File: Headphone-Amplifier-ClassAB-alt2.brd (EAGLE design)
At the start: 40.6 x 17.8 mm, 17 parts, among them T1 2N3904, T2 2N3904, T3 2N3906

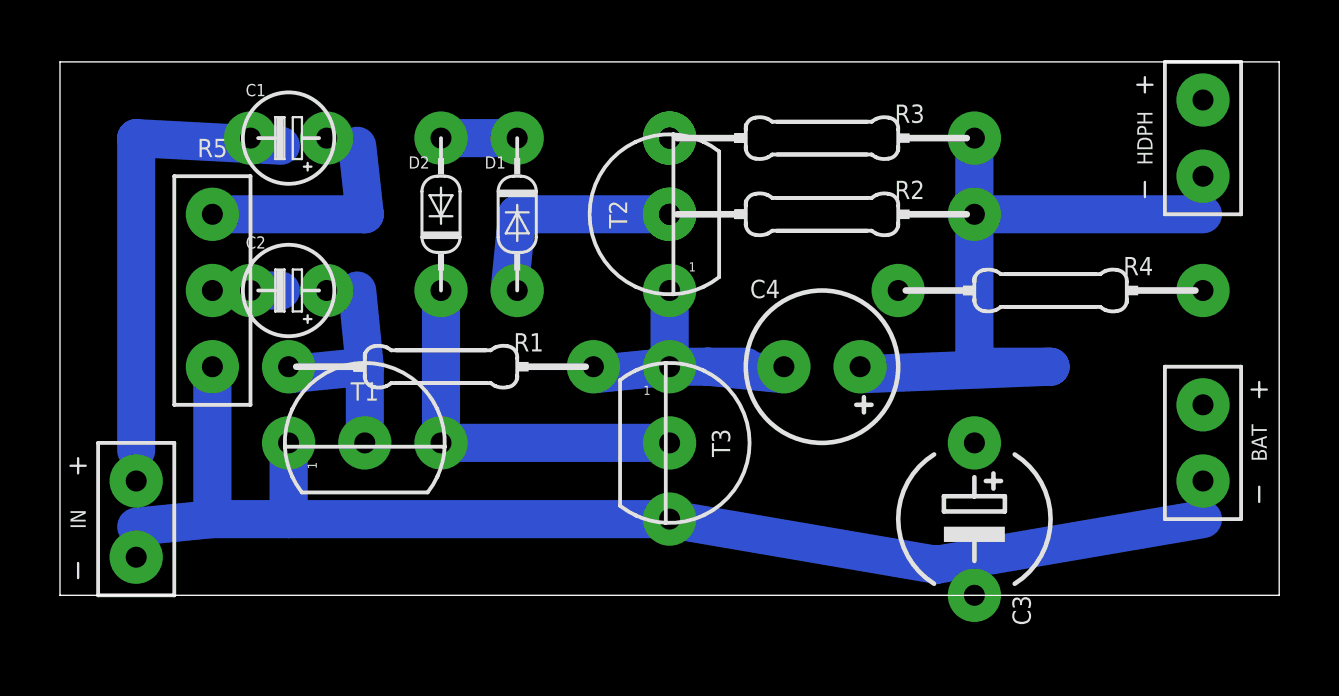
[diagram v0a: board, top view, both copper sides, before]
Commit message: ...
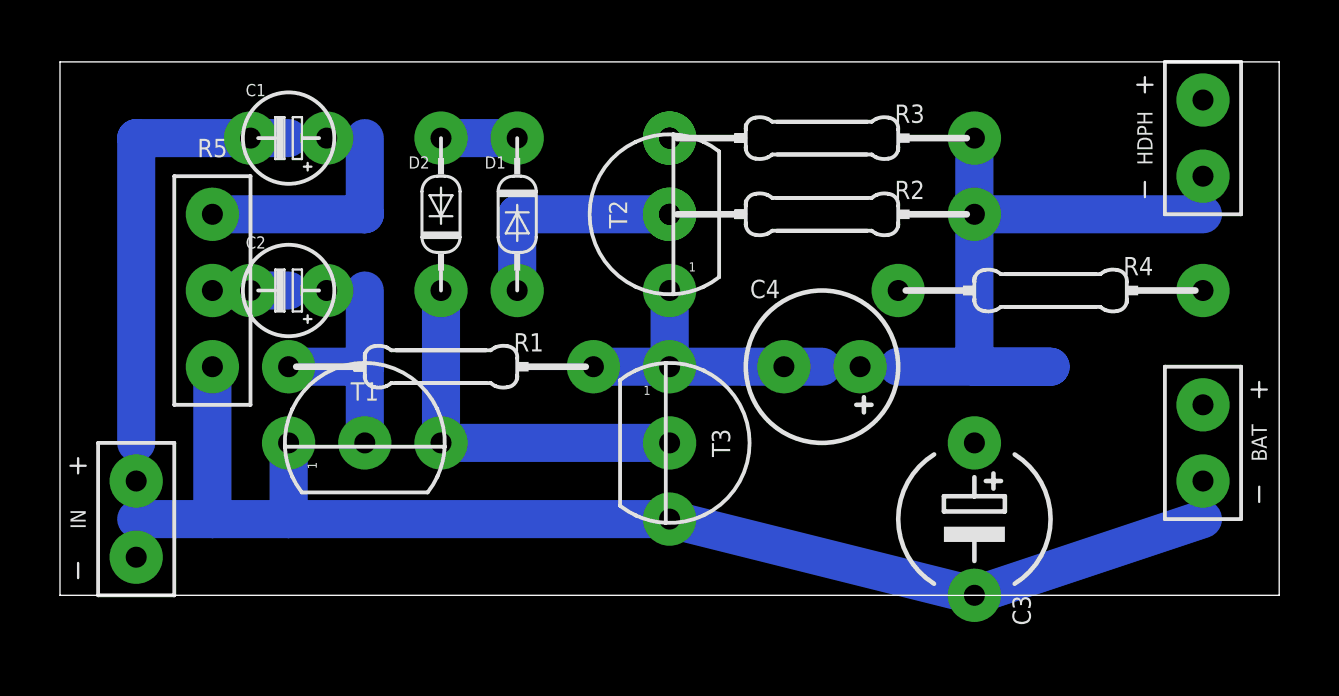
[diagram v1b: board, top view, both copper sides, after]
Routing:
- net N$9: track 23.9 -> 22.9 mm
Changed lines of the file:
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@@
           <contactref element="R2" pad="1" />
           <contactref element="T2" pad="2" />
-          <wire x1="14.986" y1="10.16" x2="15.24" y2="12.7" width="1.27" layer="16" />
+          <wire x1="15.24" y1="10.16" x2="15.24" y2="12.7" width="1.27" layer="16" />
           <wire x1="15.24" y1="12.7" x2="20.32" y2="12.7" width="1.27" layer="16" />
         </signal>
@@
           <contactref element="D2" pad="A" />
           <contactref element="D1" pad="C" />
-          <wire x1="12.7" y1="15.24" x2="14.986" y2="15.24" width="1.27" layer="16" />
+          <wire x1="12.7" y1="15.24" x2="15.24" y2="15.24" width="1.27" layer="16" />
         </signal>
         <signal name="N$4">
@@
           <contactref element="T2" pad="1" />
           <contactref element="T3" pad="1" />
-          <wire x1="17.78" y1="7.366" x2="20.32" y2="7.62" width="1.27" layer="16" />
+          <wire x1="17.78" y1="7.62" x2="20.32" y2="7.62" width="1.27" layer="16" />
           <wire x1="20.32" y1="7.62" x2="20.32" y2="10.16" width="1.27" layer="16" />
-          <wire x1="20.32" y1="7.62" x2="21.59" y2="7.62" width="1.27" layer="16" />
-          <wire x1="22.86" y1="7.62" x2="21.59" y2="7.62" width="1.27" layer="16" />
-          <wire x1="21.59" y1="7.62" x2="24.13" y2="7.366" width="1.27" layer="16" />
+          <wire x1="20.32" y1="7.62" x2="22.86" y2="7.62" width="1.27" layer="16" />
+          <wire x1="22.86" y1="7.62" x2="22.86" y2="7.62" width="1.27" layer="16" />
+          <wire x1="22.86" y1="7.62" x2="25.4" y2="7.62" width="1.27" layer="16" />
         </signal>
         <signal name="N$5">
           <contactref element="C1" pad="+" />
           <contactref element="R5" pad="3" />
-          <wire x1="9.906" y1="14.986" x2="10.16" y2="12.7" width="1.27" layer="16" />
+          <wire x1="10.16" y1="15.24" x2="10.16" y2="12.7" width="1.27" layer="16" />
           <wire x1="10.16" y1="12.7" x2="5.08" y2="12.7" width="1.27" layer="16" />
         </signal>
@@
           <contactref element="R5" pad="2" />
           <contactref element="C2" pad="-" />
-          <wire x1="5.08" y1="10.16" x2="7.366" y2="10.16" width="1.27" layer="16" />
+          <wire x1="5.08" y1="10.16" x2="7.62" y2="10.16" width="1.27" layer="16" />
         </signal>
         <signal name="N$7">
@@
           <contactref element="R1" pad="1" />
           <wire x1="10.16" y1="5.08" x2="10.16" y2="7.62" width="1.27" layer="16" />
-          <wire x1="7.62" y1="7.366" x2="10.16" y2="7.62" width="1.27" layer="16" />
-          <wire x1="10.16" y1="7.62" x2="9.906" y2="10.16" width="1.27" layer="16" />
+          <wire x1="7.62" y1="7.62" x2="10.16" y2="7.62" width="1.27" layer="16" />
+          <wire x1="10.16" y1="7.62" x2="10.16" y2="10.16" width="1.27" layer="16" />
         </signal>
         <signal name="GND">
@@
           <contactref element="IN" pad="1" />
           <contactref element="T3" pad="3" />
-          <wire x1="2.54" y1="2.286" x2="5.08" y2="2.54" width="1.27" layer="16" />
+          <wire x1="2.54" y1="2.54" x2="5.08" y2="2.54" width="1.27" layer="16" />
           <wire x1="5.08" y1="7.62" x2="5.08" y2="2.54" width="1.27" layer="16" />
           <wire x1="5.08" y1="2.54" x2="7.62" y2="2.54" width="1.27" layer="16" />
           <wire x1="7.62" y1="5.08" x2="7.62" y2="2.54" width="1.27" layer="16" />
           <wire x1="7.62" y1="2.54" x2="20.32" y2="2.54" width="1.27" layer="16" />
-          <wire x1="29.21" y1="1.016" x2="20.32" y2="2.54" width="1.27" layer="16" />
-          <wire x1="29.21" y1="1.016" x2="38.1" y2="2.54" width="1.27" layer="16" />
+          <wire x1="30.48" y1="0" x2="20.32" y2="2.54" width="1.27" layer="16" />
+          <wire x1="30.48" y1="0" x2="38.1" y2="2.54" width="1.27" layer="16" />
         </signal>
         <signal name="N$9">
@@
           <contactref element="R3" pad="2" />
           <wire x1="38.1" y1="12.7" x2="30.48" y2="12.7" width="1.27" layer="16" />
-          <wire x1="30.48" y1="12.7" x2="30.48" y2="14.986" width="1.27" layer="16" />
+          <wire x1="30.48" y1="12.7" x2="30.48" y2="15.24" width="1.27" layer="16" />
           <wire x1="30.48" y1="12.7" x2="30.48" y2="7.62" width="1.27" layer="16" />
           <wire x1="30.48" y1="7.62" x2="33.02" y2="7.62" width="1.27" layer="16" />
-          <wire x1="33.02" y1="7.62" x2="26.67" y2="7.366" width="1.27" layer="16" />
+          <wire x1="33.02" y1="7.62" x2="27.94" y2="7.62" width="1.27" layer="16" />
         </signal>
         <signal name="N$8">
@@
           <contactref element="R3" pad="1" />
           <contactref element="T2" pad="3" />
-          <wire x1="20.32" y1="15.24" x2="20.32" y2="14.986" width="1.27" layer="16" />
+          <wire x1="20.32" y1="15.24" x2="20.32" y2="15.24" width="1.27" layer="16" />
           <wire x1="27.94" y1="10.16" x2="38.1" y2="15.24" width="0" layer="19" extent="1-1" />
           <wire x1="29.21" y1="6.096" x2="27.94" y2="10.16" width="0" layer="19" extent="1-1" />
@@
           <contactref element="IN" pad="2" />
           <contactref element="C1" pad="-" />
-          <wire x1="7.366" y1="14.986" x2="2.54" y2="15.24" width="1.27" layer="16" />
-          <wire x1="2.54" y1="15.24" x2="2.54" y2="4.826" width="1.27" layer="16" />
+          <wire x1="7.62" y1="15.24" x2="2.54" y2="15.24" width="1.27" layer="16" />
+          <wire x1="2.54" y1="15.24" x2="2.54" y2="5.08" width="1.27" layer="16" />
         </signal>
       </signals>

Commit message: ...
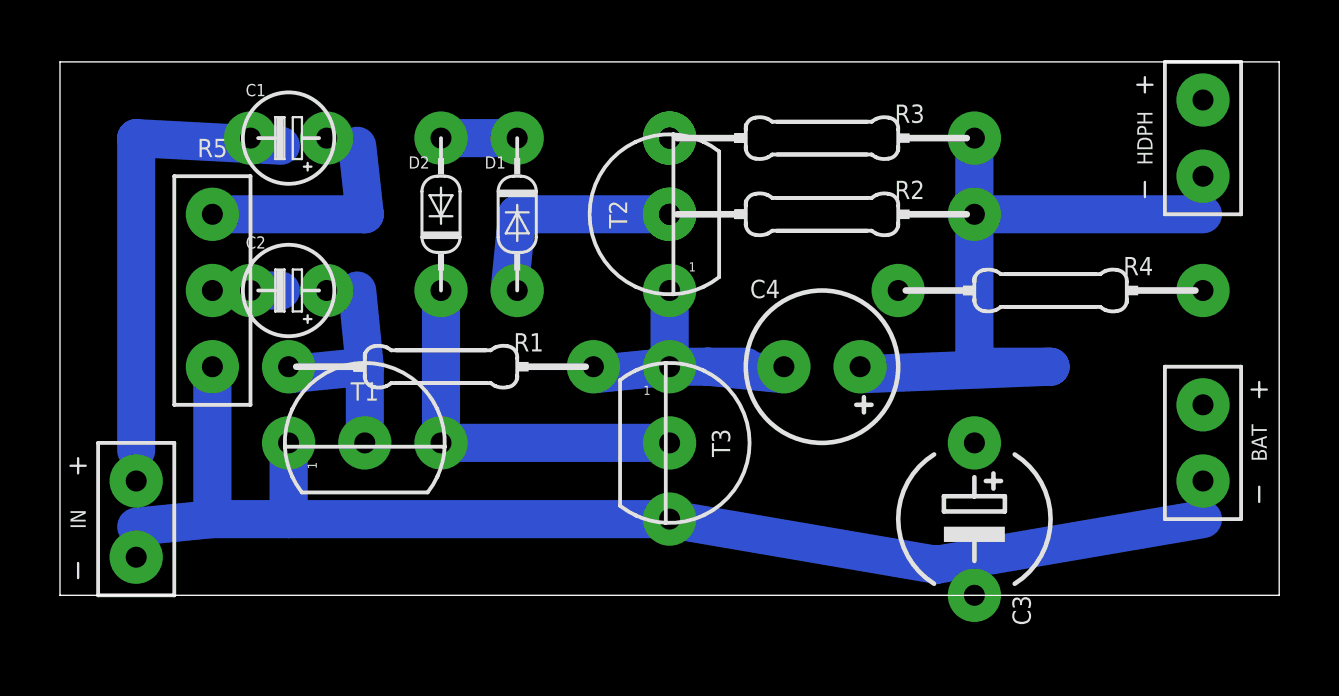
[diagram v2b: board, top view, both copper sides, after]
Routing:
- net N$9: track 22.9 -> 23.9 mm
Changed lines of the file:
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@@
           <contactref element="R2" pad="1" />
           <contactref element="T2" pad="2" />
-          <wire x1="15.24" y1="10.16" x2="15.24" y2="12.7" width="1.27" layer="16" />
+          <wire x1="14.986" y1="10.16" x2="15.24" y2="12.7" width="1.27" layer="16" />
           <wire x1="15.24" y1="12.7" x2="20.32" y2="12.7" width="1.27" layer="16" />
         </signal>
@@
           <contactref element="D2" pad="A" />
           <contactref element="D1" pad="C" />
-          <wire x1="12.7" y1="15.24" x2="15.24" y2="15.24" width="1.27" layer="16" />
+          <wire x1="12.7" y1="15.24" x2="14.986" y2="15.24" width="1.27" layer="16" />
         </signal>
         <signal name="N$4">
@@
           <contactref element="T2" pad="1" />
           <contactref element="T3" pad="1" />
-          <wire x1="17.78" y1="7.62" x2="20.32" y2="7.62" width="1.27" layer="16" />
+          <wire x1="17.78" y1="7.366" x2="20.32" y2="7.62" width="1.27" layer="16" />
           <wire x1="20.32" y1="7.62" x2="20.32" y2="10.16" width="1.27" layer="16" />
-          <wire x1="20.32" y1="7.62" x2="22.86" y2="7.62" width="1.27" layer="16" />
-          <wire x1="22.86" y1="7.62" x2="22.86" y2="7.62" width="1.27" layer="16" />
-          <wire x1="22.86" y1="7.62" x2="25.4" y2="7.62" width="1.27" layer="16" />
+          <wire x1="20.32" y1="7.62" x2="21.59" y2="7.62" width="1.27" layer="16" />
+          <wire x1="22.86" y1="7.62" x2="21.59" y2="7.62" width="1.27" layer="16" />
+          <wire x1="21.59" y1="7.62" x2="24.13" y2="7.366" width="1.27" layer="16" />
         </signal>
         <signal name="N$5">
           <contactref element="C1" pad="+" />
           <contactref element="R5" pad="3" />
-          <wire x1="10.16" y1="15.24" x2="10.16" y2="12.7" width="1.27" layer="16" />
+          <wire x1="9.906" y1="14.986" x2="10.16" y2="12.7" width="1.27" layer="16" />
           <wire x1="10.16" y1="12.7" x2="5.08" y2="12.7" width="1.27" layer="16" />
         </signal>
@@
           <contactref element="R5" pad="2" />
           <contactref element="C2" pad="-" />
-          <wire x1="5.08" y1="10.16" x2="7.62" y2="10.16" width="1.27" layer="16" />
+          <wire x1="5.08" y1="10.16" x2="7.366" y2="10.16" width="1.27" layer="16" />
         </signal>
         <signal name="N$7">
@@
           <contactref element="R1" pad="1" />
           <wire x1="10.16" y1="5.08" x2="10.16" y2="7.62" width="1.27" layer="16" />
-          <wire x1="7.62" y1="7.62" x2="10.16" y2="7.62" width="1.27" layer="16" />
-          <wire x1="10.16" y1="7.62" x2="10.16" y2="10.16" width="1.27" layer="16" />
+          <wire x1="7.62" y1="7.366" x2="10.16" y2="7.62" width="1.27" layer="16" />
+          <wire x1="10.16" y1="7.62" x2="9.906" y2="10.16" width="1.27" layer="16" />
         </signal>
         <signal name="GND">
@@
           <contactref element="IN" pad="1" />
           <contactref element="T3" pad="3" />
-          <wire x1="2.54" y1="2.54" x2="5.08" y2="2.54" width="1.27" layer="16" />
+          <wire x1="2.54" y1="2.286" x2="5.08" y2="2.54" width="1.27" layer="16" />
           <wire x1="5.08" y1="7.62" x2="5.08" y2="2.54" width="1.27" layer="16" />
           <wire x1="5.08" y1="2.54" x2="7.62" y2="2.54" width="1.27" layer="16" />
           <wire x1="7.62" y1="5.08" x2="7.62" y2="2.54" width="1.27" layer="16" />
           <wire x1="7.62" y1="2.54" x2="20.32" y2="2.54" width="1.27" layer="16" />
-          <wire x1="30.48" y1="0" x2="20.32" y2="2.54" width="1.27" layer="16" />
-          <wire x1="30.48" y1="0" x2="38.1" y2="2.54" width="1.27" layer="16" />
+          <wire x1="29.21" y1="1.016" x2="20.32" y2="2.54" width="1.27" layer="16" />
+          <wire x1="29.21" y1="1.016" x2="38.1" y2="2.54" width="1.27" layer="16" />
         </signal>
         <signal name="N$9">
@@
           <contactref element="R3" pad="2" />
           <wire x1="38.1" y1="12.7" x2="30.48" y2="12.7" width="1.27" layer="16" />
-          <wire x1="30.48" y1="12.7" x2="30.48" y2="15.24" width="1.27" layer="16" />
+          <wire x1="30.48" y1="12.7" x2="30.48" y2="14.986" width="1.27" layer="16" />
           <wire x1="30.48" y1="12.7" x2="30.48" y2="7.62" width="1.27" layer="16" />
           <wire x1="30.48" y1="7.62" x2="33.02" y2="7.62" width="1.27" layer="16" />
-          <wire x1="33.02" y1="7.62" x2="27.94" y2="7.62" width="1.27" layer="16" />
+          <wire x1="33.02" y1="7.62" x2="26.67" y2="7.366" width="1.27" layer="16" />
         </signal>
         <signal name="N$8">
@@
           <contactref element="R3" pad="1" />
           <contactref element="T2" pad="3" />
-          <wire x1="20.32" y1="15.24" x2="20.32" y2="15.24" width="1.27" layer="16" />
+          <wire x1="20.32" y1="15.24" x2="20.32" y2="14.986" width="1.27" layer="16" />
           <wire x1="27.94" y1="10.16" x2="38.1" y2="15.24" width="0" layer="19" extent="1-1" />
           <wire x1="29.21" y1="6.096" x2="27.94" y2="10.16" width="0" layer="19" extent="1-1" />
@@
           <contactref element="IN" pad="2" />
           <contactref element="C1" pad="-" />
-          <wire x1="7.62" y1="15.24" x2="2.54" y2="15.24" width="1.27" layer="16" />
-          <wire x1="2.54" y1="15.24" x2="2.54" y2="5.08" width="1.27" layer="16" />
+          <wire x1="7.366" y1="14.986" x2="2.54" y2="15.24" width="1.27" layer="16" />
+          <wire x1="2.54" y1="15.24" x2="2.54" y2="4.826" width="1.27" layer="16" />
         </signal>
       </signals>
